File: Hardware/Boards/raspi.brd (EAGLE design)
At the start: 14.9 x 30.5 mm, 4 parts

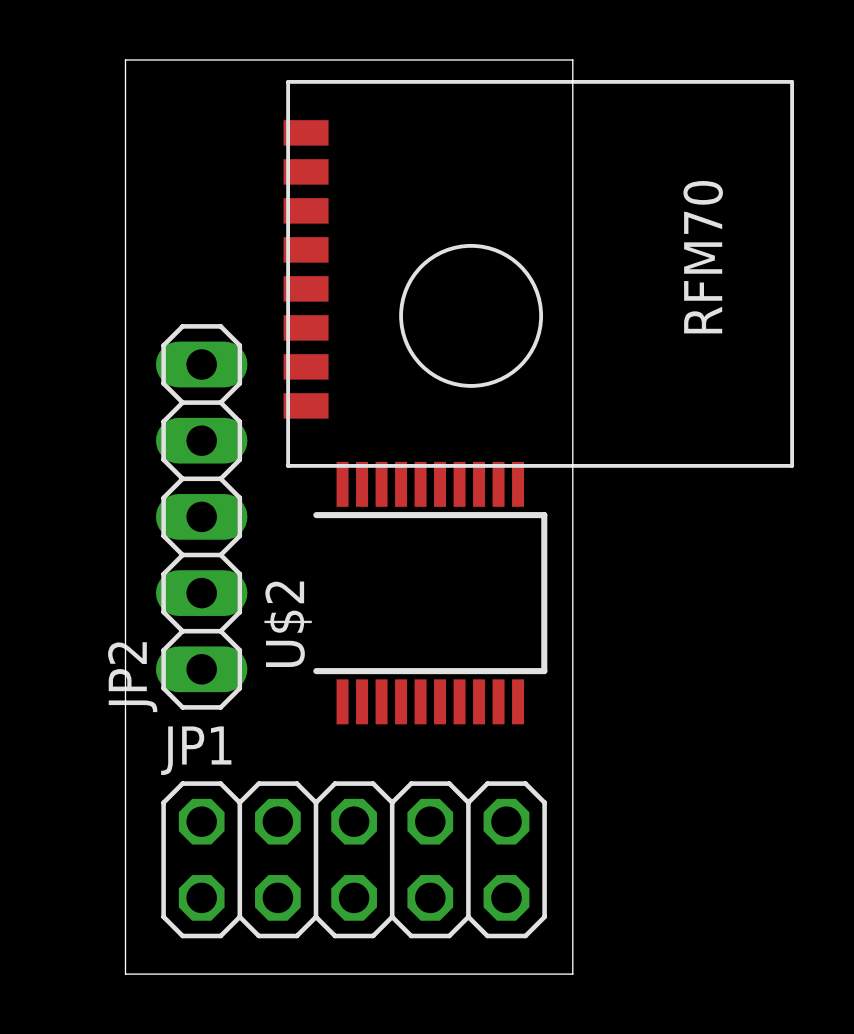
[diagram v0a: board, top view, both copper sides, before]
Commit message: a
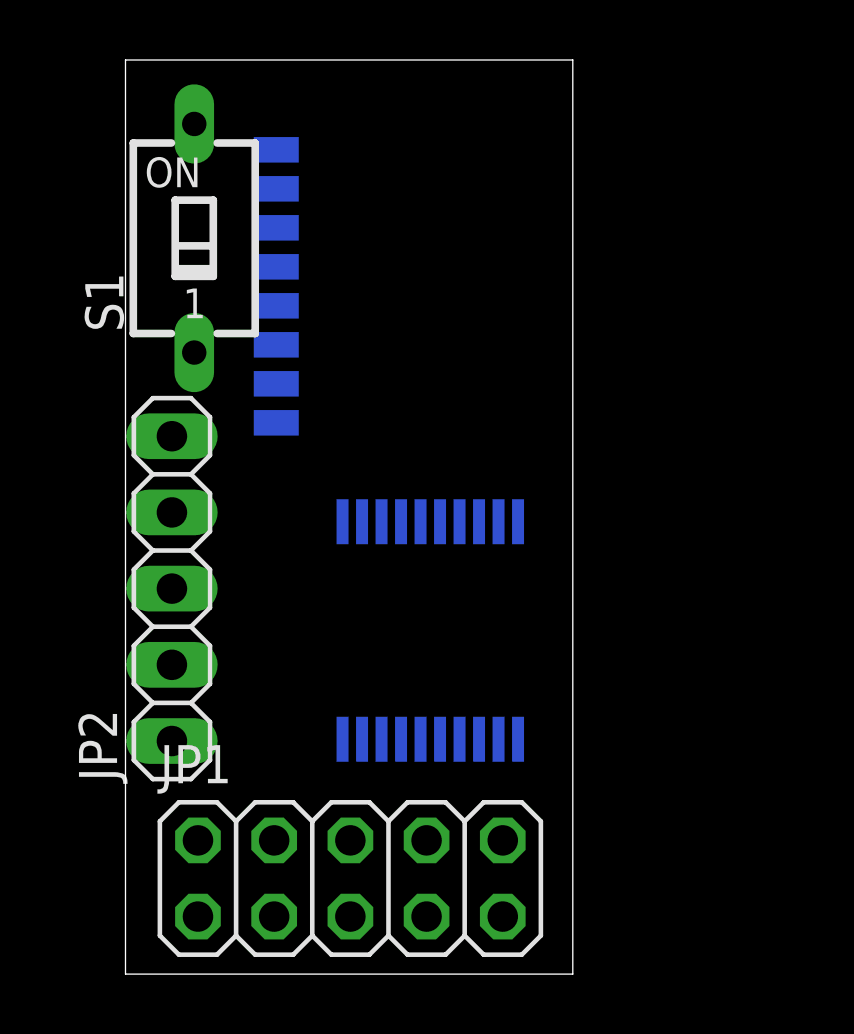
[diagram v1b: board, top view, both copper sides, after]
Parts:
- added S1: (no value), switch-dil:SD4-01
- moved U$1 9.52 mm to (19.3, 18.5), flipped to the bottom, turned to 90 degrees
- moved JP2 2.59 mm to (1.55, 12.8)
- moved U$2 1.25 mm to (10.2, 11.5), flipped to the bottom
- moved JP1 0.63 mm to (7.50, 3.19)
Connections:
- new net N$1: S1.2, U$2.2
- net N$5: now also S1.1
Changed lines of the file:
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@@
 <setting verticaltext="up"/>
 </settings>
-<grid distance="0.05" unitdist="inch" unit="inch" style="lines" multiple="1" display="no" altdistance="0.025" altunitdist="inch" altunit="inch"/>
+<grid distance="0.003125" unitdist="mic" unit="mm" style="lines" multiple="1" display="no" altdistance="0.025" altunitdist="inch" altunit="inch"/>
 <layers>
 <layer number="1" name="Top" color="4" fill="1" visible="yes" active="yes"/>
@@
 </autorouter>
 <elements>
-<element name="U$1" library="rfm70" package="RFM70" value="RFM70" x="20.32" y="27.94" rot="R270"/>
-<element name="U$2" library="microchip" package="SSOP20" value="PIC16F690" x="10.16" y="12.7"/>
-<element name="JP2" library="pinhead" package="1X05" value="Prog" x="2.54" y="15.24" rot="R90"/>
-<element name="JP1" library="pinhead" package="2X05" value="Raspi" x="7.62" y="3.81"/>
+<element name="U$1" library="rfm70" package="RFM70" value="RFM70" x="19.3274875" y="18.475259375" rot="MR90"/>
+<element name="U$2" library="microchip" package="SSOP20" value="PIC16F690" x="10.16" y="11.4546375" rot="MR0"/>
+<element name="JP2" library="pinhead" package="1X05" value="Prog" x="1.547484375" y="12.849175" rot="R90"/>
+<element name="JP1" library="pinhead" package="2X05" value="Raspi" x="7.495934375" y="3.18731875"/>
+<element name="S1" library="switch-dil" package="SD4-01" value="" x="2.291871875" y="24.528246875">
+<attribute name="OC_NEWARK" value="unknown" x="2.291871875" y="24.528246875" size="1.778" layer="27" display="off"/>
+<attribute name="MPN" value="" x="2.291871875" y="24.528246875" size="1.778" layer="27" display="off"/>
+<attribute name="MF" value="" x="2.291871875" y="24.528246875" size="1.778" layer="27" display="off"/>
+<attribute name="OC_FARNELL" value="unknown" x="2.291871875" y="24.528246875" size="1.778" layer="27" display="off"/>
+</element>
 </elements>
 <signals>
@@
 <contactref element="JP2" pad="3"/>
 <contactref element="JP1" pad="6"/>
-<wire x1="7.235" y1="16.325" x2="6.02" y2="28.04" width="0" layer="19" extent="1-1"/>
-<wire x1="7.62" y1="5.08" x2="7.235" y2="16.325" width="0" layer="19" extent="1-1"/>
-<wire x1="2.54" y1="15.24" x2="7.62" y2="5.08" width="0" layer="19" extent="1-1"/>
+<contactref element="S1" pad="1"/>
+<wire x1="13.085" y1="15.0796375" x2="5.0274875" y2="18.375259375" width="0" layer="19" extent="1-1"/>
+<wire x1="1.547484375" y1="12.849175" x2="13.085" y2="15.0796375" width="0" layer="19" extent="1-1"/>
+<wire x1="7.495934375" y1="4.45731875" x2="13.085" y2="15.0796375" width="0" layer="19" extent="1-1"/>
+<wire x1="2.291871875" y1="20.718246875" x2="7.495934375" y2="4.45731875" width="0" layer="19" extent="1-1"/>
 </signal>
 <signal name="N$12">
 <contactref element="U$1" pad="MISO"/>
 <contactref element="U$2" pad="13"/>
-<wire x1="11.785" y1="16.325" x2="6.02" y2="20.24" width="0" layer="19" extent="1-1"/>
+<wire x1="8.535" y1="15.0796375" x2="5.0274875" y2="26.175259375" width="0" layer="19" extent="1-1"/>
 </signal>
 <signal name="N$17">
@@
 <contactref element="JP2" pad="2"/>
 <contactref element="JP1" pad="1"/>
-<wire x1="7.235" y1="9.075" x2="6.02" y2="26.74" width="0" layer="19" extent="1-1"/>
-<wire x1="2.54" y1="2.54" x2="7.235" y2="9.075" width="0" layer="19" extent="1-1"/>
-<wire x1="2.54" y1="12.7" x2="2.54" y2="2.54" width="0" layer="19" extent="1-1"/>
+<wire x1="13.085" y1="7.8296375" x2="5.0274875" y2="19.675259375" width="0" layer="19" extent="1-1"/>
+<wire x1="2.415934375" y1="1.91731875" x2="13.085" y2="7.8296375" width="0" layer="19" extent="1-1"/>
+<wire x1="1.547484375" y1="10.309175" x2="2.415934375" y2="1.91731875" width="0" layer="19" extent="1-1"/>
 </signal>
 <signal name="N$18">
 <contactref element="U$2" pad="19"/>
 <contactref element="JP2" pad="4"/>
-<wire x1="7.885" y1="16.325" x2="2.54" y2="17.78" width="0" layer="19" extent="1-1"/>
+<wire x1="12.435" y1="15.0796375" x2="1.547484375" y2="15.389175" width="0" layer="19" extent="1-1"/>
 </signal>
 <signal name="N$19">
 <contactref element="U$2" pad="18"/>
 <contactref element="JP2" pad="5"/>
-<wire x1="8.535" y1="16.325" x2="2.54" y2="20.32" width="0" layer="19" extent="1-1"/>
+<wire x1="11.785" y1="15.0796375" x2="1.547484375" y2="17.929175" width="0" layer="19" extent="1-1"/>
 </signal>
 <signal name="N$16">
 <contactref element="U$2" pad="17"/>
 <contactref element="U$1" pad="CE"/>
-<wire x1="9.185" y1="16.325" x2="6.02" y2="25.44" width="0" layer="19" extent="1-1"/>
+<wire x1="11.135" y1="15.0796375" x2="5.0274875" y2="20.975259375" width="0" layer="19" extent="1-1"/>
 </signal>
 <signal name="N$20">
 <contactref element="U$2" pad="16"/>
 <contactref element="U$1" pad="CSN"/>
-<wire x1="9.835" y1="16.325" x2="6.02" y2="24.14" width="0" layer="19" extent="1-1"/>
+<wire x1="10.485" y1="15.0796375" x2="5.0274875" y2="22.275259375" width="0" layer="19" extent="1-1"/>
 </signal>
 <signal name="N$21">
 <contactref element="U$2" pad="14"/>
 <contactref element="U$1" pad="IRQ"/>
-<wire x1="11.135" y1="16.325" x2="6.02" y2="18.94" width="0" layer="19" extent="1-1"/>
+<wire x1="9.185" y1="15.0796375" x2="5.0274875" y2="27.475259375" width="0" layer="19" extent="1-1"/>
 </signal>
 <signal name="N$22">
 <contactref element="U$2" pad="11"/>
 <contactref element="U$1" pad="SCK"/>
-<wire x1="13.085" y1="16.325" x2="6.02" y2="22.84" width="0" layer="19" extent="1-1"/>
+<wire x1="7.235" y1="15.0796375" x2="5.0274875" y2="23.575259375" width="0" layer="19" extent="1-1"/>
 </signal>
 <signal name="N$23">
 <contactref element="U$2" pad="9"/>
 <contactref element="U$1" pad="MOSI"/>
-<wire x1="12.435" y1="9.075" x2="6.02" y2="21.54" width="0" layer="19" extent="1-1"/>
+<wire x1="7.885" y1="7.8296375" x2="5.0274875" y2="24.875259375" width="0" layer="19" extent="1-1"/>
 </signal>
 <signal name="N$25">
 <contactref element="U$2" pad="4"/>
 <contactref element="JP2" pad="1"/>
-<wire x1="9.185" y1="9.075" x2="2.54" y2="10.16" width="0" layer="19" extent="1-1"/>
+<wire x1="11.135" y1="7.8296375" x2="1.547484375" y2="7.769175" width="0" layer="19" extent="1-1"/>
 </signal>
 <signal name="N$28">
@@
 <contactref element="U$2" pad="10"/>
 <contactref element="JP1" pad="10"/>
-<wire x1="13.085" y1="9.075" x2="12.7" y2="5.08" width="0" layer="19" extent="1-1"/>
+<wire x1="7.235" y1="7.8296375" x2="12.575934375" y2="4.45731875" width="0" layer="19" extent="1-1"/>
 </signal>
 <signal name="N$34">
 <contactref element="U$2" pad="12"/>
 <contactref element="JP1" pad="8"/>
-<wire x1="12.435" y1="16.325" x2="10.16" y2="5.08" width="0" layer="19" extent="1-1"/>
+<wire x1="7.885" y1="15.0796375" x2="10.035934375" y2="4.45731875" width="0" layer="19" extent="1-1"/>
+</signal>
+<signal name="N$1">
+<contactref element="S1" pad="2"/>
+<contactref element="U$2" pad="2"/>
+<wire x1="2.291871875" y1="28.338246875" x2="12.435" y2="7.8296375" width="0" layer="19" extent="1-1"/>
 </signal>
 </signals>
